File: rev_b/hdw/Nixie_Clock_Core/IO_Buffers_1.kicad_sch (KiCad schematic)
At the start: 8 parts

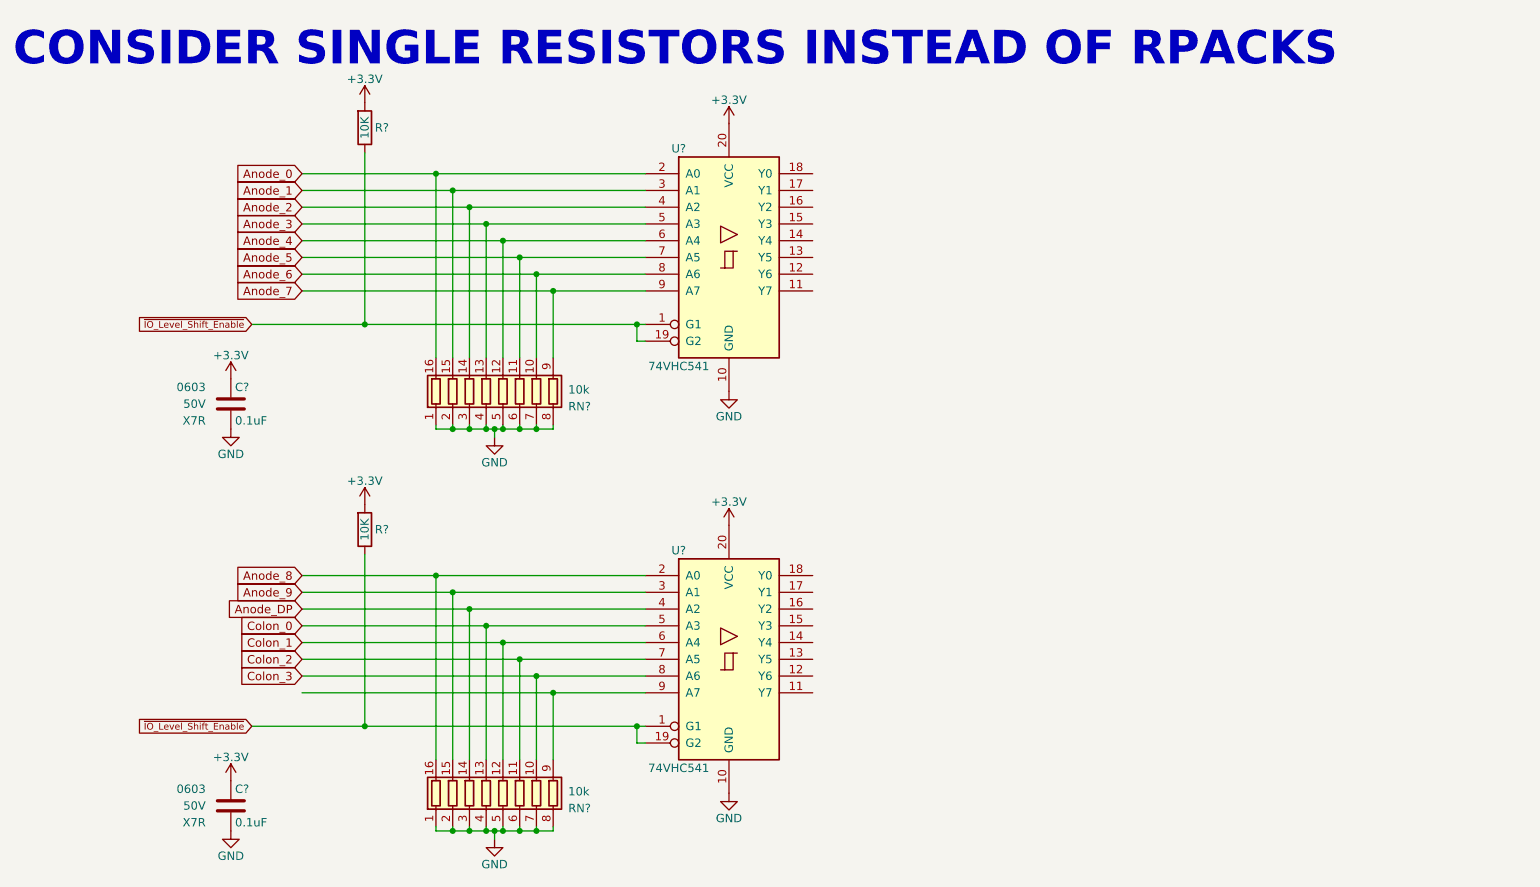
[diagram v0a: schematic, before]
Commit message: more rev b sch progress
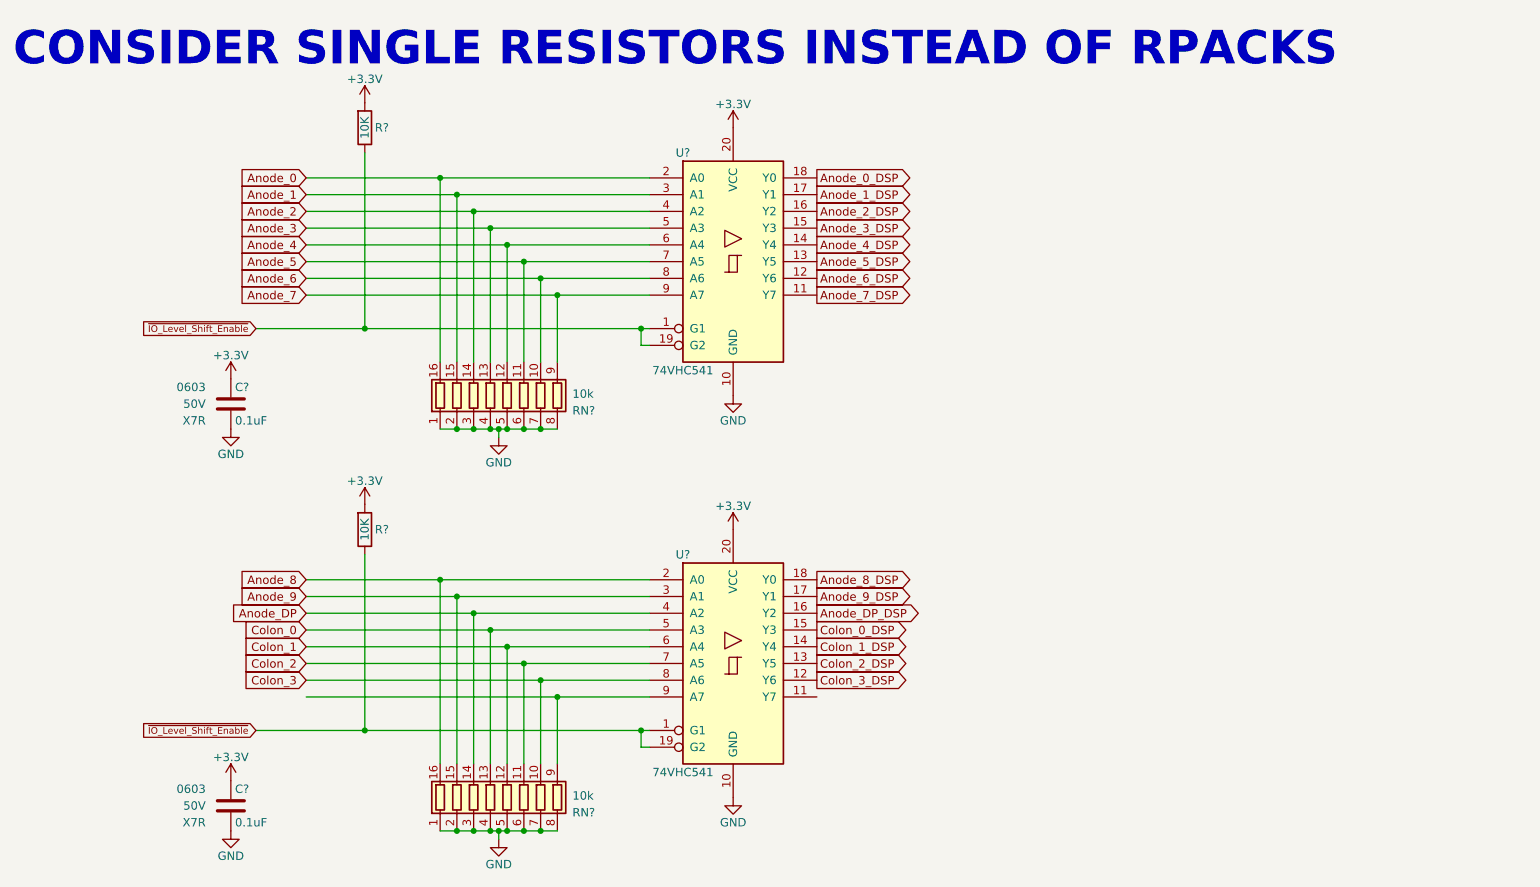
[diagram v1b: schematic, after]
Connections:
- net Anode_7_DSP: now reaches U?.11 (Y7)
- net Anode_6_DSP: now reaches U?.12 (Y6)
- net Anode_5_DSP: now reaches U?.13 (Y5)
- net Anode_4_DSP: now reaches U?.14 (Y4)
- net Anode_3_DSP: now reaches U?.15 (Y3)
- net Anode_2_DSP: now reaches U?.16 (Y2)
- net Anode_1_DSP: now reaches U?.17 (Y1)
- net Anode_0_DSP: now reaches U?.18 (Y0)
- net Colon_3_DSP: now reaches U?.12 (Y6)
- net Colon_2_DSP: now reaches U?.13 (Y5)
- net Colon_1_DSP: now reaches U?.14 (Y4)
- net Colon_0_DSP: now reaches U?.15 (Y3)
- net Anode_DP_DSP: now reaches U?.16 (Y2)
- net Anode_9_DSP: now reaches U?.17 (Y1)
- net Anode_8_DSP: now reaches U?.18 (Y0)
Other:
- moved on the sheet: RN?, U?
